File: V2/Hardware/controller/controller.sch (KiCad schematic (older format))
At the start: 31 parts, among them J0 Molex_PSU_F, J1 4pins_jumper, J2 Flat_7seg_F, J3 Rpi_DATA_F, Q0 BD139-16, Q1 BD139-16, Q2 BD139-16, Q3 BD139-16, Q4 BD139-16, Q5 BD139-16, Q6 BD139-16, U1 ATtiny2313-20PU

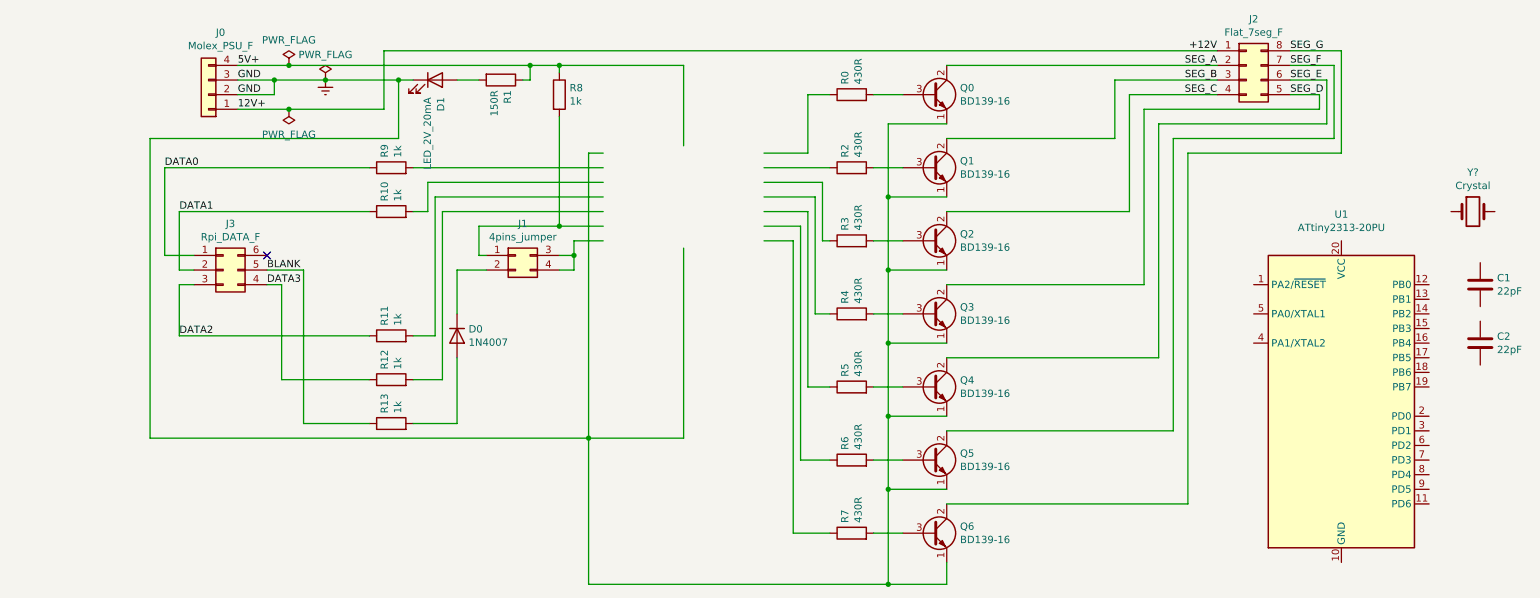
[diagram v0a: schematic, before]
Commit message: Update schematics
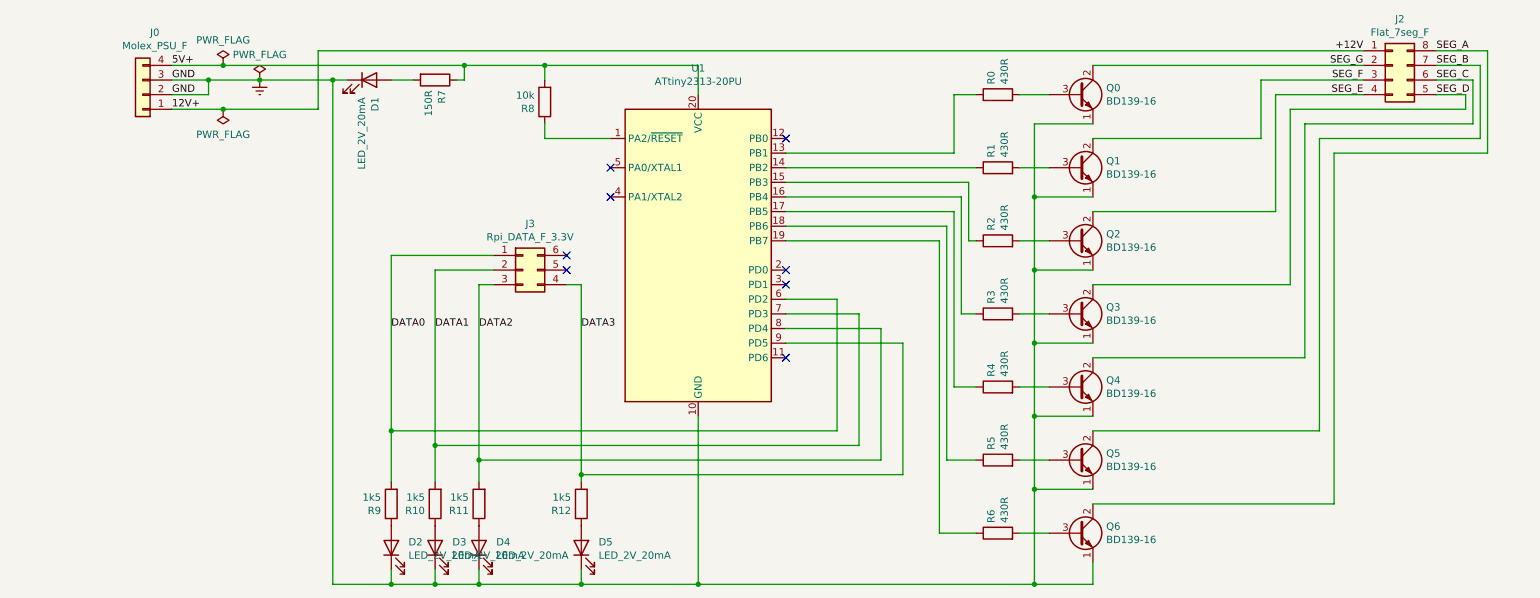
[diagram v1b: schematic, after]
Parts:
- removed C1, C2: 22pF, symbol Device:C
- removed D0: 1N4007, Diode_THT:D_A-405_P10.16mm_Horizontal, symbol Device:D
- removed J1: 4pins_jumper, Connector_PinHeader_2.00mm:PinHeader_2x02_P2.00mm_Vertical, symbol Connector_Generic:Conn_02x02_Top_Bottom
- removed R13: 1k, Resistor_THT:R_Axial_DIN0207_L6.3mm_D2.5mm_P10.16mm_Horizontal, symbol Device:R
- removed Y?: Crystal, symbol Device:Crystal
- added D2, D3, D4, D5: LED_2V_20mA, LED_THT:LED_D5.0mm, symbol Device:LED
- J3: value Rpi_DATA_F -> Rpi_DATA_F_3.3V
- R10, R11, R12, R9: value 1k -> 1k5
- R8: value 1k -> 10k
- renumbered R2 to R1, R3 to R2, R4 to R3, R5 to R4, R6 to R5, R7 to R6, R1 to R7
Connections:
- net labels removed: BLANK
- wire segments 135 -> 124
- no-connect marks 1 -> 8
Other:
- moved on the sheet: D1, J0, J2, J3, Q0, Q1, Q2, Q3, Q4, Q5, Q6, R0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

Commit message: update schemas
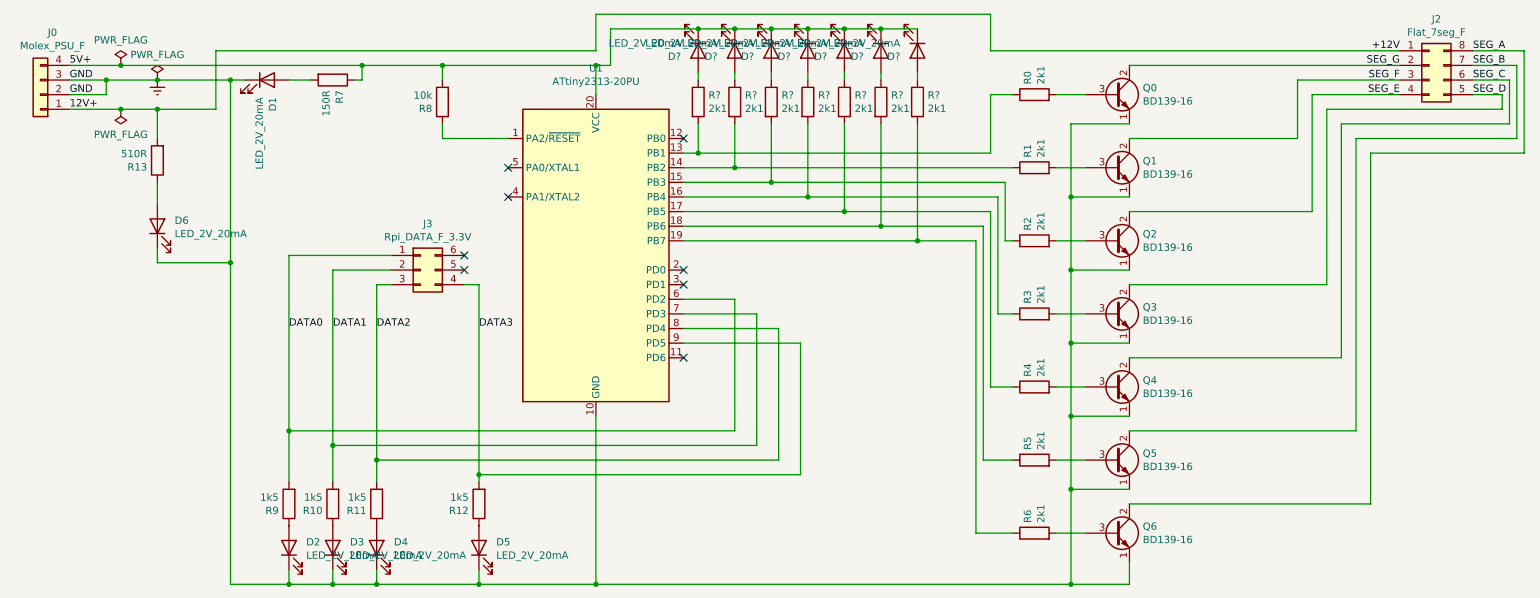
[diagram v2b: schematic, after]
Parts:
- added D6, D? (x7): LED_2V_20mA, LED_THT:LED_D5.0mm, symbol Device:LED
- added R13: 510R, Resistor_THT:R_Axial_DIN0207_L6.3mm_D2.5mm_P10.16mm_Horizontal, symbol Device:R
- added R? (x7): 2k1, Resistor_THT:R_Axial_DIN0207_L6.3mm_D2.5mm_P10.16mm_Horizontal, symbol Device:R
- R0, R1, R2, R3, R4, R5, R6: value 430R -> 2k1
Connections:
- net +12V: now also R13.2
- net 5V+: now also D?.1 (K), D?.1 (K), D?.1 (K), D?.1 (K), D?.1 (K), D?.1 (K), D?.1 (K)
- net Earth: now also D6.1 (K)
- net at R0.1, U1.13 (PB1): now also R?.2
- net at R1.1, U1.14 (PB2): now also R?.2
- net at R2.1, U1.15 (PB3): now also R?.2
- net at R3.1, U1.16 (PB4): now also R?.2
- net at R4.1, U1.17 (PB5): now also R?.2
- net at R5.1, U1.18 (PB6): now also R?.2
- net at R6.1, U1.19 (PB7): now also R?.2
- new net: D6.2 (A), R13.1
- new net: D?.2 (A), R?.1 (x7)
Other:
- moved on the sheet: D1, D2, D3, D4, D5, J0, J2, J3, Q0, Q1, Q2, Q3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
